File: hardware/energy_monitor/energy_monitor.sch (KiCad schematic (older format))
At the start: 46 parts, among them J1 Screw_Terminal_01x03, U1 RAC04, U2 ADS131E08

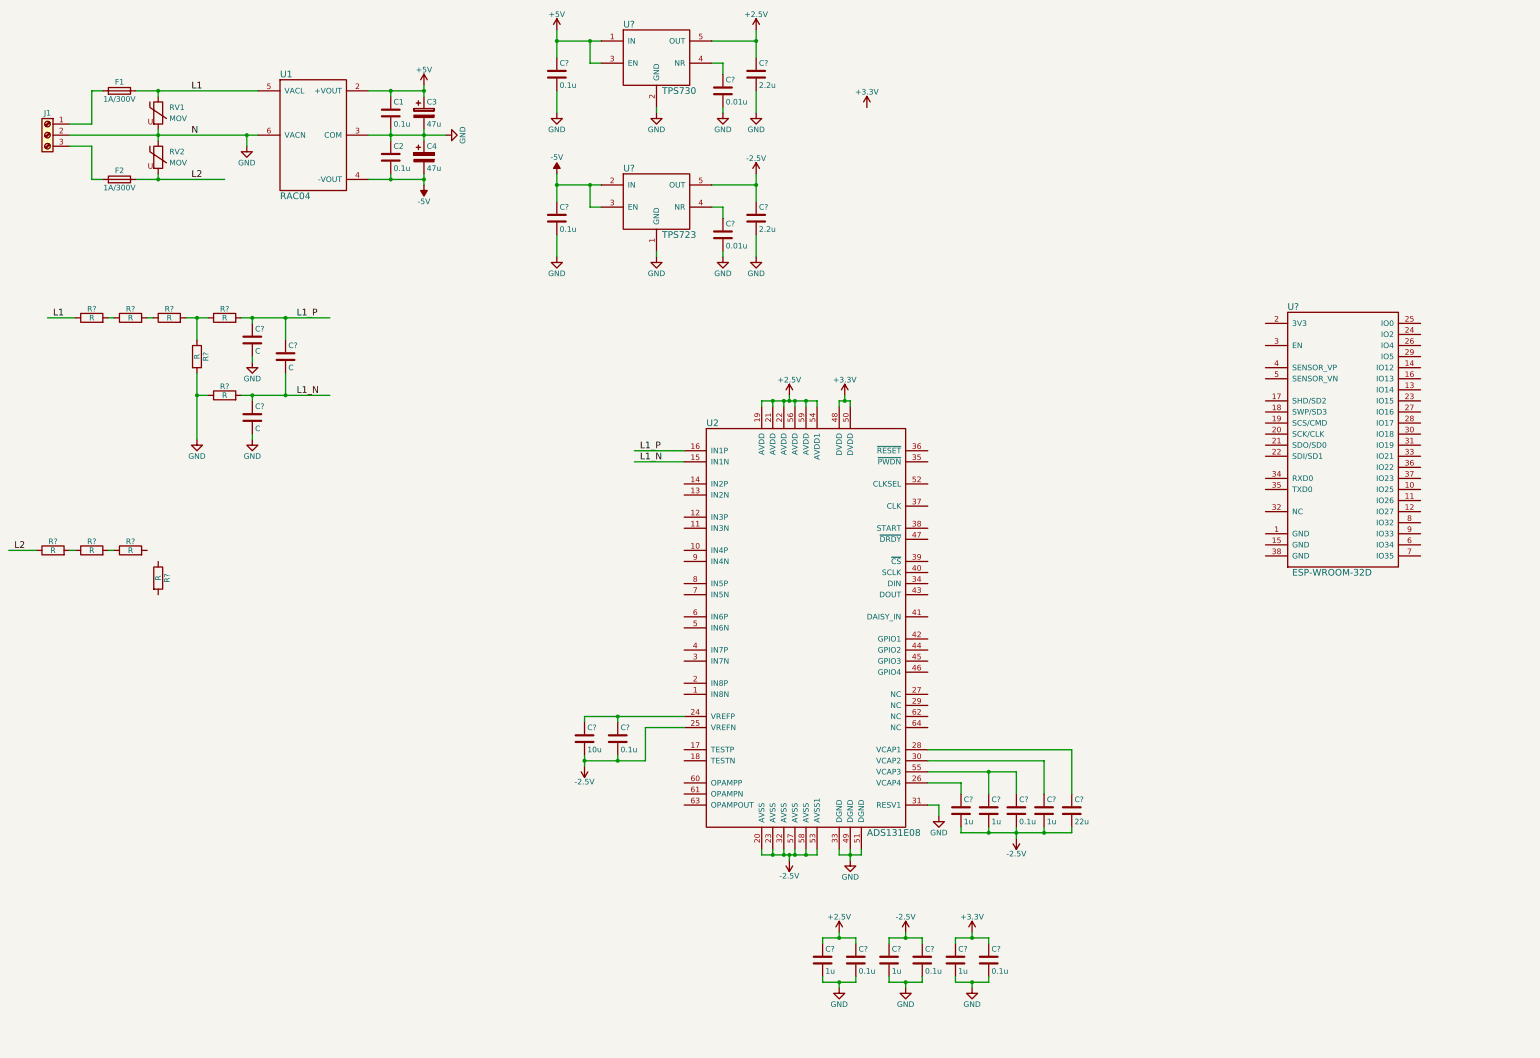
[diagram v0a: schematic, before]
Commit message: Working on schematic
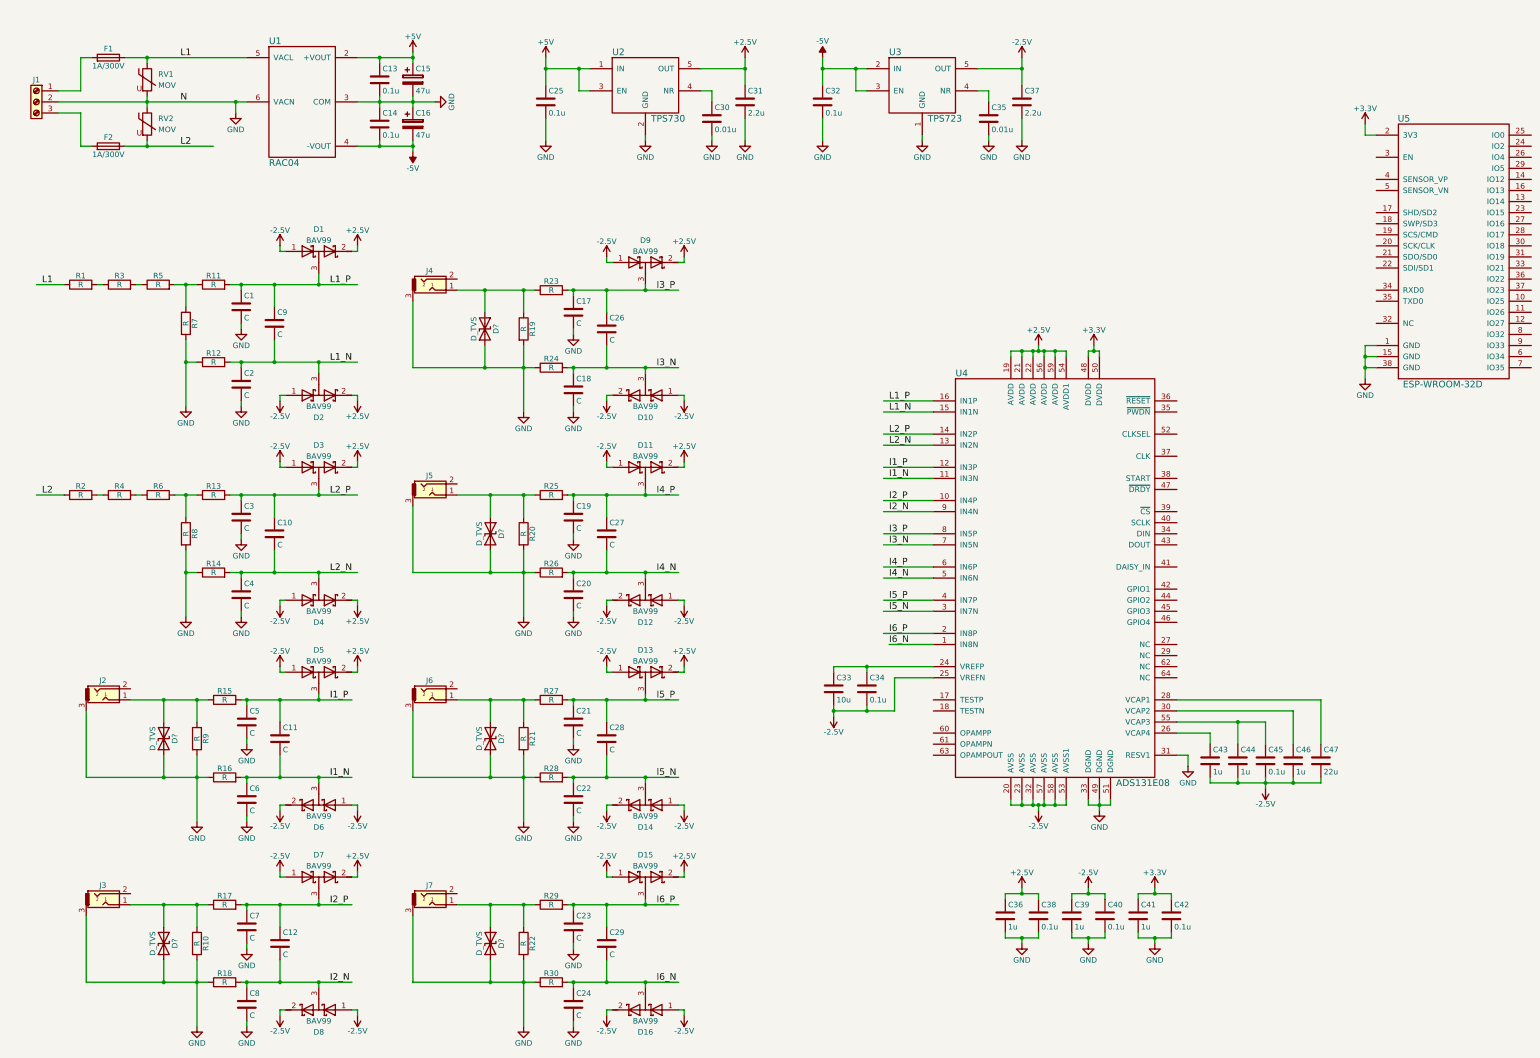
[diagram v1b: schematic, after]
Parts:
- added C10, C11, C12, C17, C18, C19, C20, C21, C22, C23, C24, C26, C27, C28, C29, C3, C4, C5, C6, C7, C8: C, symbol C
- added D1, D10, D11, D12, D13, D14, D15, D16, D2, D3, D4, D5, D6, D7, D8, D9: BAV99, symbol D_Schottky_x2_Serial_AKC
- added D? (x6): D_TVS, symbol D_TVS
- added J2, J3, J4, J5, J6, J7: Audio-Jack-3, symbol Audio-Jack-3
- added R10, R13, R14, R15, R16, R17, R18, R19, R20, R21, R22, R23, R24, R25, R26, R27, R28, R29, R30, R9: R, symbol R
- gave numbers to parts that had none: 35
- renumbered C1 to C13, C2 to C14, C3 to C15, C4 to C16, U2 to U4
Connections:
- net labels added: I1_N, I1_P, I2_N, I2_P, I3_N, I3_P, I4_N, I4_P, I5_N, I5_P, I6_N, I6_P, L2_N, L2_P
- wire segments 139 -> 341
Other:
- moved on the sheet: C1, C13, C14, C15, C16, C2, C25, C30, C31, C32, C33, C34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
